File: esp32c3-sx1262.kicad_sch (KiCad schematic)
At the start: 36 parts, among them J1 HDR-M-2.54_1x4, J3 HDR-M-2.54_1x1, J4 HDR-M-2.54_1x2, U1 -, U3 SKY13330-397LF, U4 XC6220B331MR, U5 IPEX-1, X3 32MHz

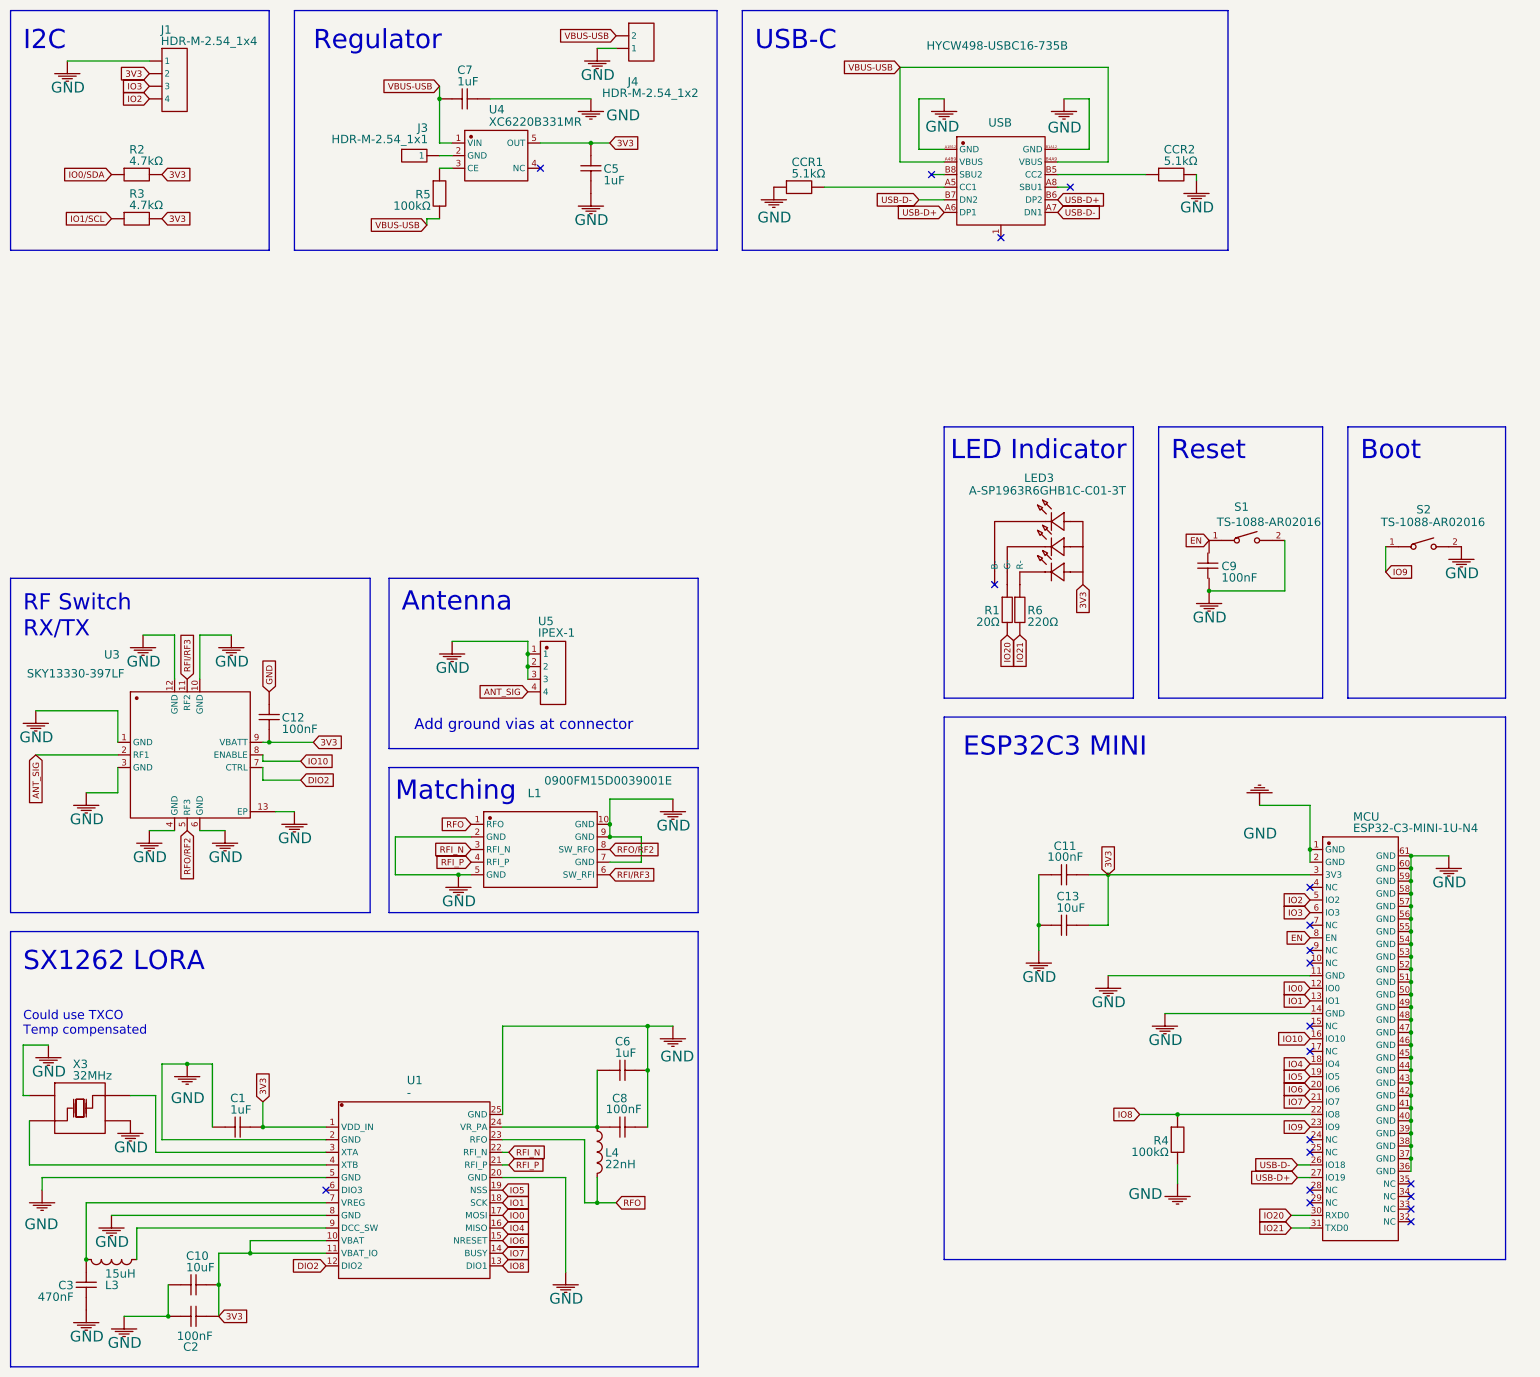
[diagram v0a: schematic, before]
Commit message: Add files via upload
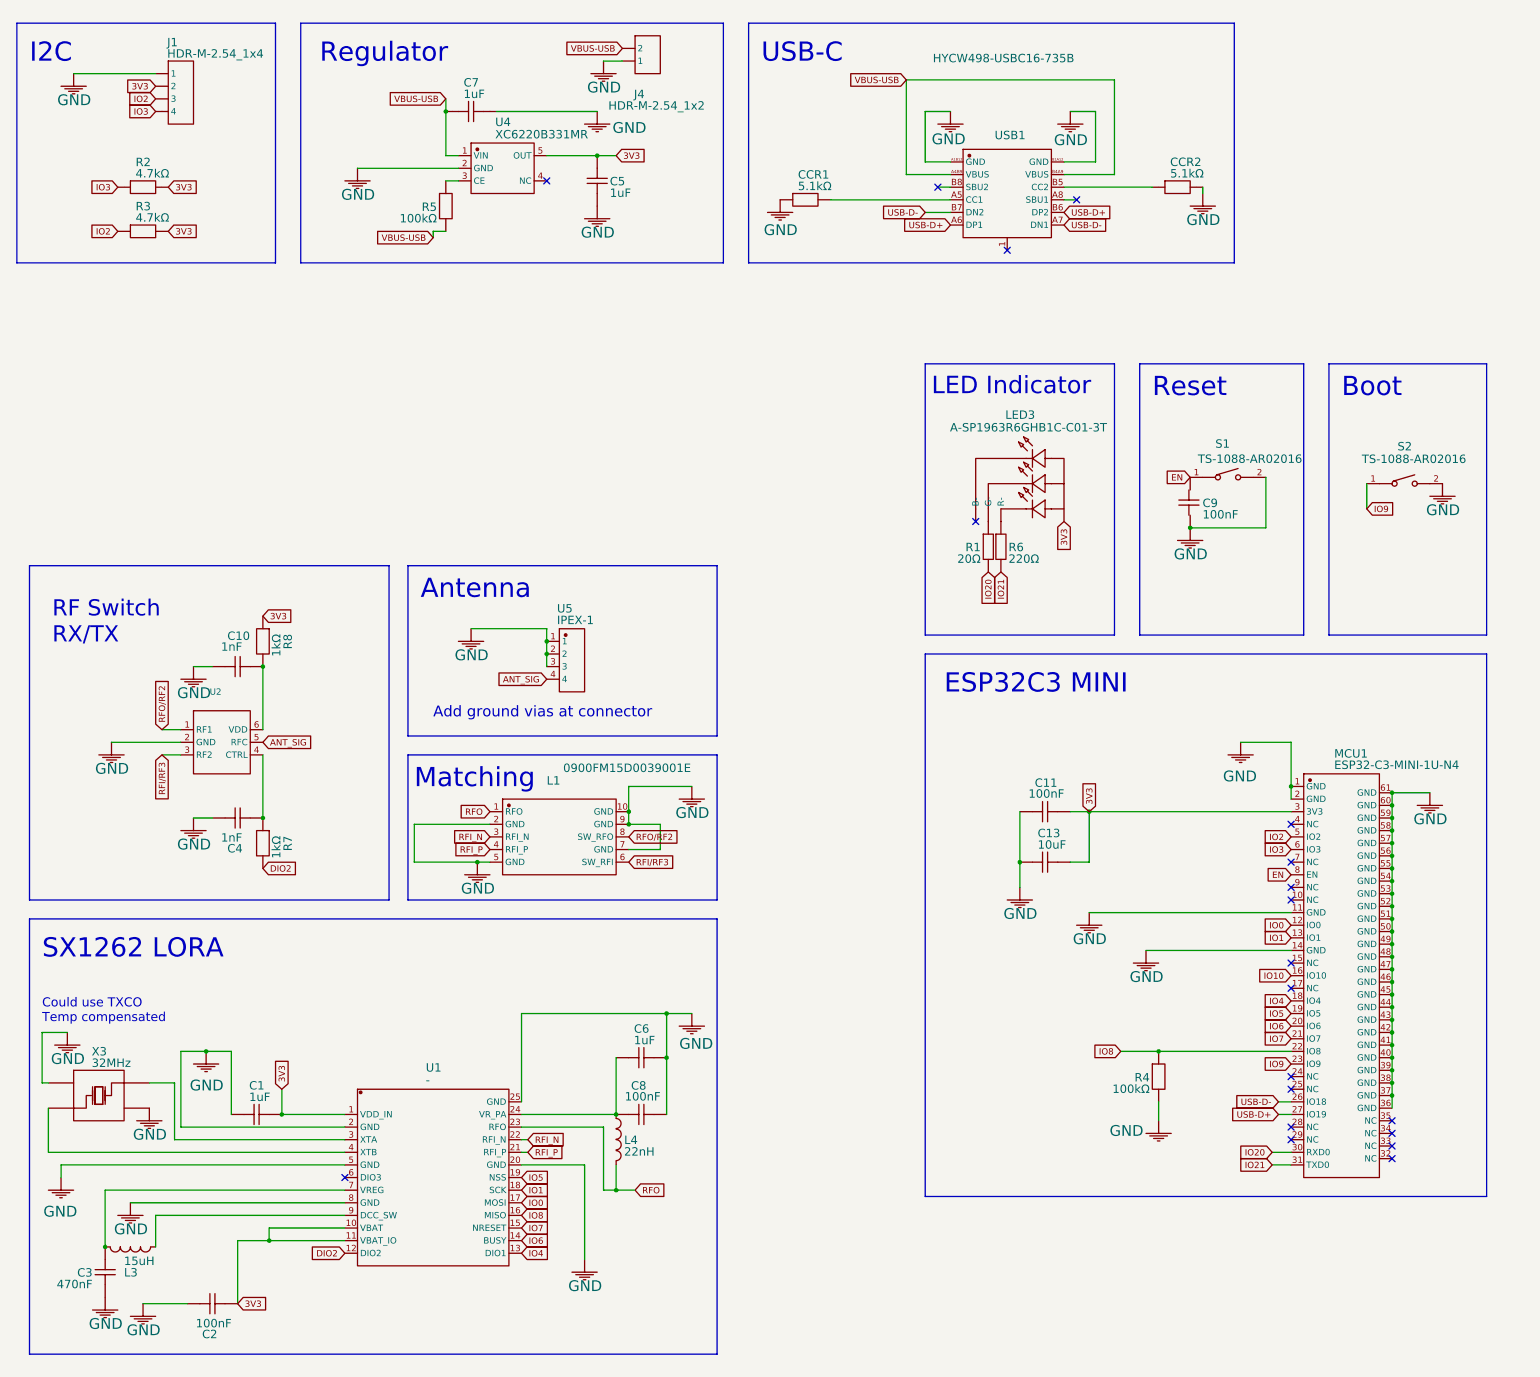
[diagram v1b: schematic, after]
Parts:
- removed C10: 10uF, symbol CL10A106MA8NRNC_1
- removed C12: 100nF, symbol FCC0402B104K160AT
- removed J3: HDR-M-2.54_1x1, symbol HDR-M-2.54_1x1
- removed U3: SKY13330-397LF, symbol SKY13330-397LF
- added C10, C4: 1nF, Library:C0603, symbol CC0603KRX7R9BB104_2
- added R7, R8: 1kΩ, Library:R0603, symbol FRC0603F5101TS_1
- added U2: ~, Library:PE4259, symbol New_Library:PE4259
- C1, C11, C13, C2, C3, C5, C6, C7, C8, C9: footprint (none) -> Library:C0603
- CCR1, CCR2, R1, R2, R3, R4, R5, R6: footprint (none) -> Library:R0603
- J1: footprint (none) -> Library:HDR-M-2.54_1X4
- J4: footprint (none) -> Library:HDR-M-2.54_1X2
- L1: footprint (none) -> Library:FILTER-SMD_10P-L2.0-W1.3-BL
- L3, L4: footprint (none) -> Library:L0603
- LED3: footprint (none) -> Library:LED-SMD_4P-L1.6-W0.8_A-SP1963R6GHB1C-C01-3T
- MCU1: renamed from MCU; footprint (none) -> Library:WIFIM-SMD_61P-L13.2-W12.5-P0.80
- S1, S2: footprint (none) -> Library:SW-SMD_L3.9-W3.0-P4.45
- U1: footprint (none) -> Library:QFN-24_L4.0-W4.0-P0.50-BL-EP2.6
- U4: footprint (none) -> Library:SOT-23-5_L2.9-W1.6-P0.95-LS2.8-BR
- U5: footprint (none) -> Library:IPEX-SMD_4P-L2.6-W2.6-LS3.0
- USB1: renamed from USB; footprint (none) -> Library:USB-C-SMD_HYCW498-USBC16-735B
- X3: footprint (none) -> Library:CRYSTAL-SMD_4P-L3.2-W2.5-BL
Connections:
- net IO0/SDA is gone; now on net IO3: R2.1
- net IO1/SCL is gone; now on net IO2: R3.1
- net 3V3: now also R8.1
- net ANT_SIG: now also U2.5 (RFC)
- net DIO2: now also R7.2
- net GND: now also U4.2 (GND), C10.2, C4.2, U2.2 (GND)
- net IO2: now also J1.3; no longer J1.4
- net IO3: now also J1.4; no longer J1.3
- net IO4: now also U1.13 (DIO1); no longer U1.16 (MISO)
- net IO6: now also U1.14 (BUSY); no longer U1.15 (NRESET)
- net IO7: now also U1.15 (NRESET); no longer U1.14 (BUSY)
- net IO8: now also U1.16 (MISO); no longer U1.13 (DIO1)
- net RFI/RF3: now also U2.3 (RF2)
- net RFO/RF2: now also U2.1 (RF1)
- new net: C10.1, R8.2, U2.6 (VDD)
- new net: C4.1, R7.1, U2.4 (CTRL)
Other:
- moved on the sheet: C1, C11, C13, C2, C3, C5, C6, C7, C8, C9, CCR1, CCR2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
